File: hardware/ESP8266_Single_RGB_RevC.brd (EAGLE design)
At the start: 72.1 x 55.2 mm, 47 parts, among them IC1 ESP-12E/F, IC3 LM2594, J1 POWER_JACKPTH_LOCK, J2 B G R +, J4 G S V, Q1 IRF520, Q2 IRF520, Q3 IRF520, T1 2N3904, T2 2N3904, T3 2N3904, T4 2N3904, T5 2N3904, T6 2N3904

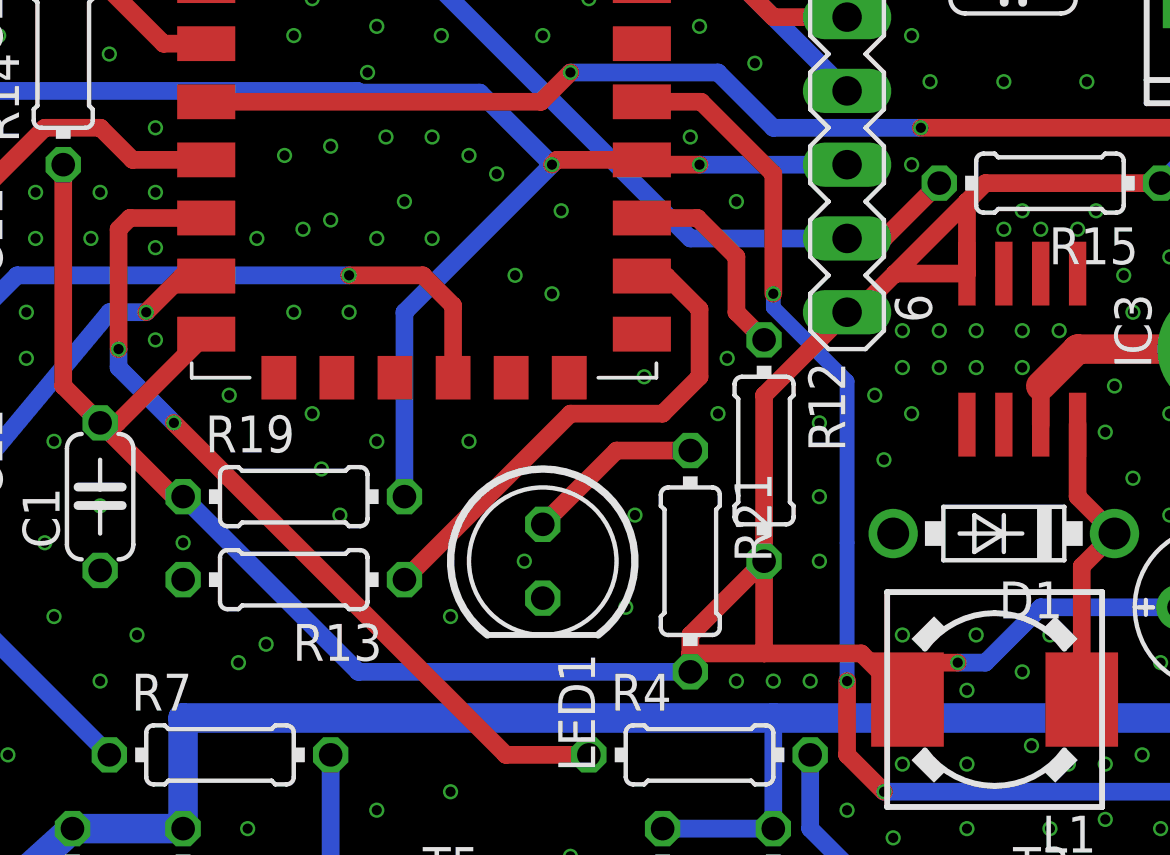
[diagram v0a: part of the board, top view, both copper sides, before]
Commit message: RevC Ok
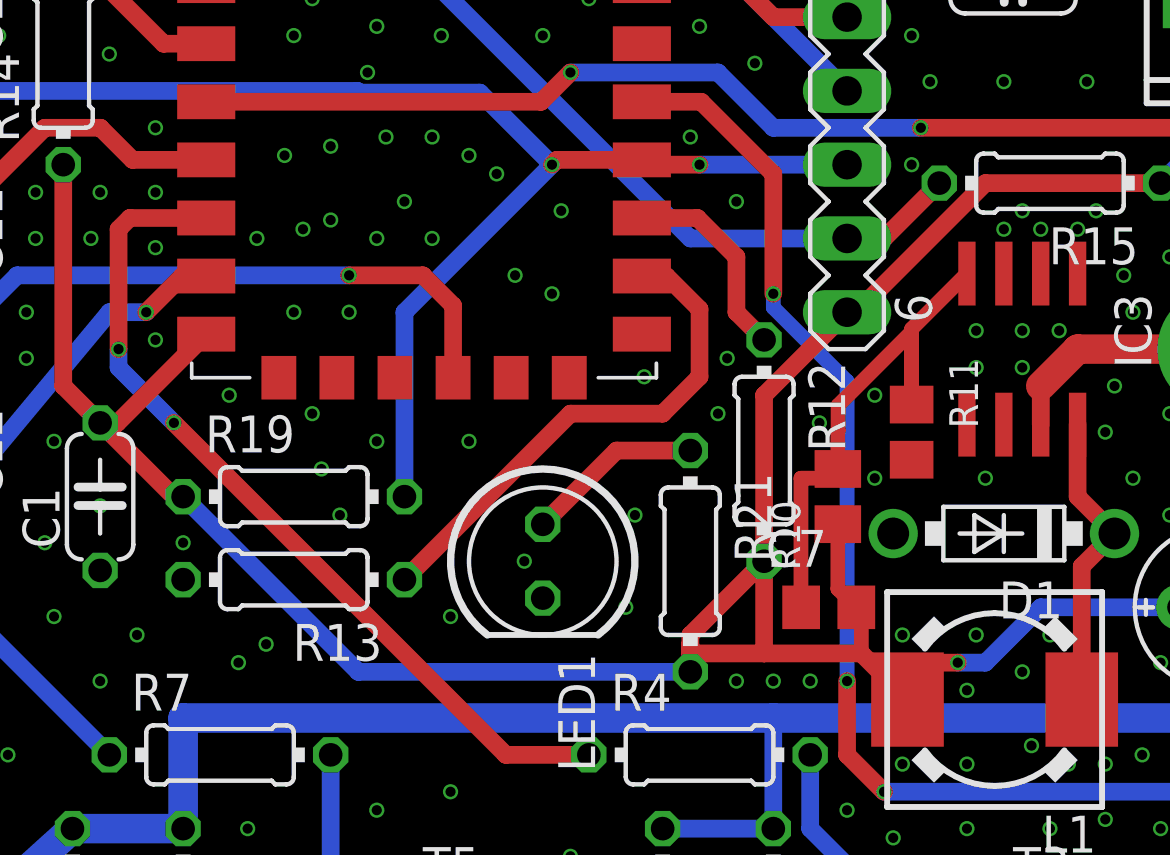
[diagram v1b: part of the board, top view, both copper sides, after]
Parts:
- added C7: 4.7n, rcl:C0805
- added R10: 1.5k, rcl:M0805
- added R11: 910, rcl:R0805
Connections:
- new net N$5: C7.1, IC3.4, R10.2, R11.1
- net +3V3: now also C7.2, R10.1; no longer IC3.4
- net GND: now also R11.2
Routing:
- net N$5: track 0.00 -> 19.4 mm
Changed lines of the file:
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@@
 <drawing>
 <settings>
-<setting alwaysvectorfont="no"/>
+<setting alwaysvectorfont="yes"/>
 <setting verticaltext="up"/>
 </settings>
@@
 <param name="mlMinCreamFrame" value="0mil"/>
 <param name="mlMaxCreamFrame" value="0mil"/>
-<param name="mlViaStopLimit" value="0mil"/>
+<param name="mlViaStopLimit" value="15mil"/>
 <param name="srRoundness" value="0"/>
 <param name="srMinRoundness" value="0mil"/>
@@
 <attribute name="POPULARITY" value="0" x="50.8" y="27.305" size="1.778" layer="27" rot="R180" display="off"/>
 </element>
+<element name="R10" library="rcl" library_urn="urn:adsk.eagle:library:334" package="M0805" package3d_urn="urn:adsk.eagle:package:23556/2" value="1.5k" x="45.4025" y="34.2925" smashed="yes" rot="R90">
+<attribute name="NAME" x="44.1071" y="31.7525" size="0.9906" layer="25" ratio="10" rot="R90"/>
+<attribute name="POPULARITY" value="45" x="45.4025" y="34.2925" size="1.778" layer="27" rot="R90" display="off"/>
+<attribute name="SPICEPREFIX" value="R" x="45.4025" y="34.2925" size="1.778" layer="27" rot="R90" display="off"/>
+<attribute name="VALUE" x="45.8851" y="32.6669" size="0.9906" layer="27" ratio="10" rot="R90"/>
+</element>
+<element name="R11" library="rcl" library_urn="urn:adsk.eagle:library:334" package="R0805" package3d_urn="urn:adsk.eagle:package:23553/2" value="910" x="47.9425" y="36.51" smashed="yes" rot="R270">
+<attribute name="NAME" x="49.2379" y="39.05" size="0.9906" layer="25" ratio="10" rot="R270"/>
+<attribute name="POPULARITY" value="86" x="47.9425" y="36.51" size="1.778" layer="27" rot="R270" display="off"/>
+<attribute name="SPICEPREFIX" value="R" x="47.9425" y="36.51" size="1.778" layer="27" rot="R270" display="off"/>
+<attribute name="VALUE" x="47.4599" y="38.1356" size="0.9906" layer="27" ratio="10" rot="R270"/>
+</element>
+<element name="C7" library="rcl" library_urn="urn:adsk.eagle:library:334" package="C0805" package3d_urn="urn:adsk.eagle:package:23617/2" value="4.7n" x="45.0875" y="30.48" smashed="yes">
+<attribute name="NAME" x="42.9285" y="31.877" size="1.27" layer="25" ratio="10"/>
+<attribute name="POPULARITY" value="88" x="45.0875" y="30.48" size="1.778" layer="27" display="off"/>
+<attribute name="SPICEPREFIX" value="C" x="45.0875" y="30.48" size="1.778" layer="27" display="off"/>
+<attribute name="VALUE" x="42.9285" y="27.813" size="1.27" layer="27" ratio="10"/>
+</element>
 </elements>
 <signals>
@@
 <via x="51.7525" y="38.735" extent="1-16" drill="0.35"/>
 <via x="50.165" y="38.735" extent="1-16" drill="0.35"/>
-<via x="48.895" y="40.005" extent="1-16" drill="0.35"/>
-<via x="48.895" y="38.735" extent="1-16" drill="0.35"/>
-<via x="47.625" y="38.735" extent="1-16" drill="0.35"/>
-<via x="47.625" y="40.005" extent="1-16" drill="0.35"/>
 <via x="46.6725" y="37.7825" extent="1-16" drill="0.35"/>
-<via x="47.9425" y="37.1475" extent="1-16" drill="0.35"/>
-<via x="46.99" y="35.56" extent="1-16" drill="0.35"/>
+<via x="50.4825" y="34.925" extent="1-16" drill="0.35"/>
+<via x="46.6725" y="34.925" extent="1-16" drill="0.35"/>
 <via x="44.7675" y="36.83" extent="1-16" drill="0.35"/>
-<via x="44.7675" y="34.29" extent="1-16" drill="0.35"/>
-<via x="44.7675" y="32.0675" extent="1-16" drill="0.35"/>
 <via x="54.9275" y="38.1" extent="1-16" drill="0.35"/>
 <via x="56.8325" y="37.1475" extent="1-16" drill="0.35"/>
@@
 <via x="22.86" y="17.78" extent="1-16" drill="0.35"/>
 <contactref element="J1" pad="GND"/>
+<contactref element="R11" pad="2"/>
 </signal>
 <signal name="N$2">
@@
 <contactref element="R15" pad="1"/>
 <contactref element="C2" pad="+"/>
-<contactref element="R21" pad="2"/>
-<contactref element="IC3" pad="4"/>
 <wire x1="57.6072" y1="51.435" x2="57.6072" y2="48.5775" width="0.6096" layer="16"/>
 <wire x1="57.6072" y1="48.5775" x2="57.6072" y2="46.1772" width="0.6096" layer="16"/>
@@
 <wire x1="56.515" y1="45.085" x2="50.4825" y2="45.085" width="0.6096" layer="1"/>
 <wire x1="46.0375" y1="40.64" x2="45.72" y2="40.64" width="0.6096" layer="1"/>
-<wire x1="50.4825" y1="45.085" x2="49.8475" y2="44.45" width="0.6096" layer="1"/>
-<wire x1="46.0375" y1="40.64" x2="47.3675" y2="41.97" width="0.6096" layer="1"/>
-<wire x1="40.3225" y1="28.2575" x2="40.3225" y2="28.8925" width="0.6096" layer="1"/>
-<wire x1="40.3225" y1="28.8925" x2="40.3225" y2="29.5275" width="0.6096" layer="1"/>
+<wire x1="40.3225" y1="28.8925" x2="40.3225" y2="29.21" width="0.6096" layer="1"/>
+<wire x1="40.3225" y1="29.21" x2="40.3225" y2="29.5275" width="0.6096" layer="1"/>
 <wire x1="40.3225" y1="29.5275" x2="42.8625" y2="32.0675" width="0.6096" layer="1"/>
 <wire x1="22.86" y1="34.29" x2="22.5425" y2="34.29" width="0.6096" layer="1"/>
@@
 <wire x1="18.7325" y1="45.72" x2="18.7325" y2="38.1" width="0.6096" layer="1"/>
 <wire x1="18.7325" y1="38.1" x2="20.0025" y2="36.83" width="0.6096" layer="1"/>
-<wire x1="40.3225" y1="28.2575" x2="28.8925" y2="28.2575" width="0.6096" layer="16"/>
-<wire x1="28.8925" y1="28.2575" x2="22.86" y2="34.29" width="0.6096" layer="16"/>
+<wire x1="22.86" y1="34.29" x2="28.8925" y2="28.2575" width="0.6096" layer="16"/>
 <contactref element="L1" pad="2"/>
 <wire x1="47.8" y1="27.305" x2="47.7125" y2="27.3925" width="0.6096" layer="1"/>
 <wire x1="47.7125" y1="27.3925" x2="46.2125" y2="28.8925" width="0.6096" layer="1"/>
-<wire x1="46.2125" y1="28.8925" x2="42.8625" y2="28.8925" width="0.6096" layer="1"/>
+<wire x1="42.8625" y1="28.8925" x2="46.2125" y2="28.8925" width="0.6096" layer="1"/>
 <wire x1="42.8625" y1="32.0675" x2="42.8625" y2="28.8925" width="0.6096" layer="1"/>
 <wire x1="57.15" y1="30.48" x2="52.3875" y2="30.48" width="0.6096" layer="16"/>
@@
 <wire x1="48.895" y1="28.575" x2="47.7125" y2="27.3925" width="0.6096" layer="1"/>
 <wire x1="42.8625" y1="28.8925" x2="40.3225" y2="28.8925" width="0.6096" layer="1"/>
-<wire x1="47.3675" y1="41.97" x2="49.8475" y2="41.97" width="0.6096" layer="1"/>
-<wire x1="49.8475" y1="41.97" x2="49.8475" y2="44.45" width="0.6096" layer="1"/>
-<wire x1="49.8475" y1="44.45" x2="47.3675" y2="41.97" width="0.6096" layer="1"/>
+<wire x1="50.4825" y1="45.085" x2="46.0375" y2="40.64" width="0.6096" layer="1"/>
+<contactref element="R10" pad="1"/>
+<contactref element="R21" pad="2"/>
+<contactref element="C7" pad="2"/>
+<wire x1="45.4025" y1="33.3425" x2="45.4025" y2="31.115" width="0.508" layer="1"/>
+<wire x1="45.4025" y1="31.115" x2="46.0375" y2="30.48" width="0.508" layer="1"/>
+<wire x1="46.2125" y1="28.8925" x2="46.2125" y2="30.305" width="0.508" layer="1"/>
+<wire x1="46.2125" y1="30.305" x2="46.0375" y2="30.48" width="0.508" layer="1"/>
+<wire x1="40.3225" y1="29.21" x2="40.3225" y2="28.2575" width="0.6096" layer="1"/>
+<wire x1="28.8925" y1="28.2575" x2="40.3225" y2="28.2575" width="0.6096" layer="16"/>
 </signal>
 <signal name="N$10">
@@
 <wire x1="53.8" y1="31.8925" x2="54.9275" y2="33.02" width="0.6096" layer="1"/>
 </signal>
+<signal name="N$5">
+<contactref element="R10" pad="2"/>
+<contactref element="R11" pad="1"/>
+<contactref element="IC3" pad="4"/>
+<contactref element="C7" pad="1"/>
+<wire x1="49.8475" y1="41.97" x2="47.9425" y2="40.065" width="0.508" layer="1"/>
+<wire x1="47.9425" y1="40.065" x2="47.9425" y2="37.46" width="0.508" layer="1"/>
+<wire x1="47.9425" y1="37.46" x2="47.9425" y2="39.96255" width="0.508" layer="1"/>
+<wire x1="45.411" y1="36.56345" x2="45.4025" y2="36.55495" width="0.508" layer="1"/>
+<wire x1="45.4025" y1="36.55495" x2="45.4025" y2="35.2425" width="0.508" layer="1"/>
+<wire x1="47.9425" y1="39.96255" x2="45.411" y2="37.43105" width="0.508" layer="1"/>
+<wire x1="45.411" y1="37.43105" x2="45.411" y2="36.56345" width="0.508" layer="1"/>
+<wire x1="45.4025" y1="35.2425" x2="45.085" y2="34.925" width="0.508" layer="1"/>
+<wire x1="45.085" y1="34.925" x2="44.1325" y2="34.925" width="0.508" layer="1"/>
+<wire x1="44.1325" y1="34.925" x2="44.1325" y2="30.485" width="0.508" layer="1"/>
+<wire x1="44.1325" y1="30.485" x2="44.1375" y2="30.48" width="0.508" layer="1"/>
+</signal>
 </signals>
